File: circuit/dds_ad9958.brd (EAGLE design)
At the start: 84 x 40.5 mm, 68 parts, among them IC1 TPS76833, IC2 TPS79318, IC3 TPS79318, IC4 AD9958, Q1 25MHz, X2 BU-SMA-V, X3 BU-SMA-V

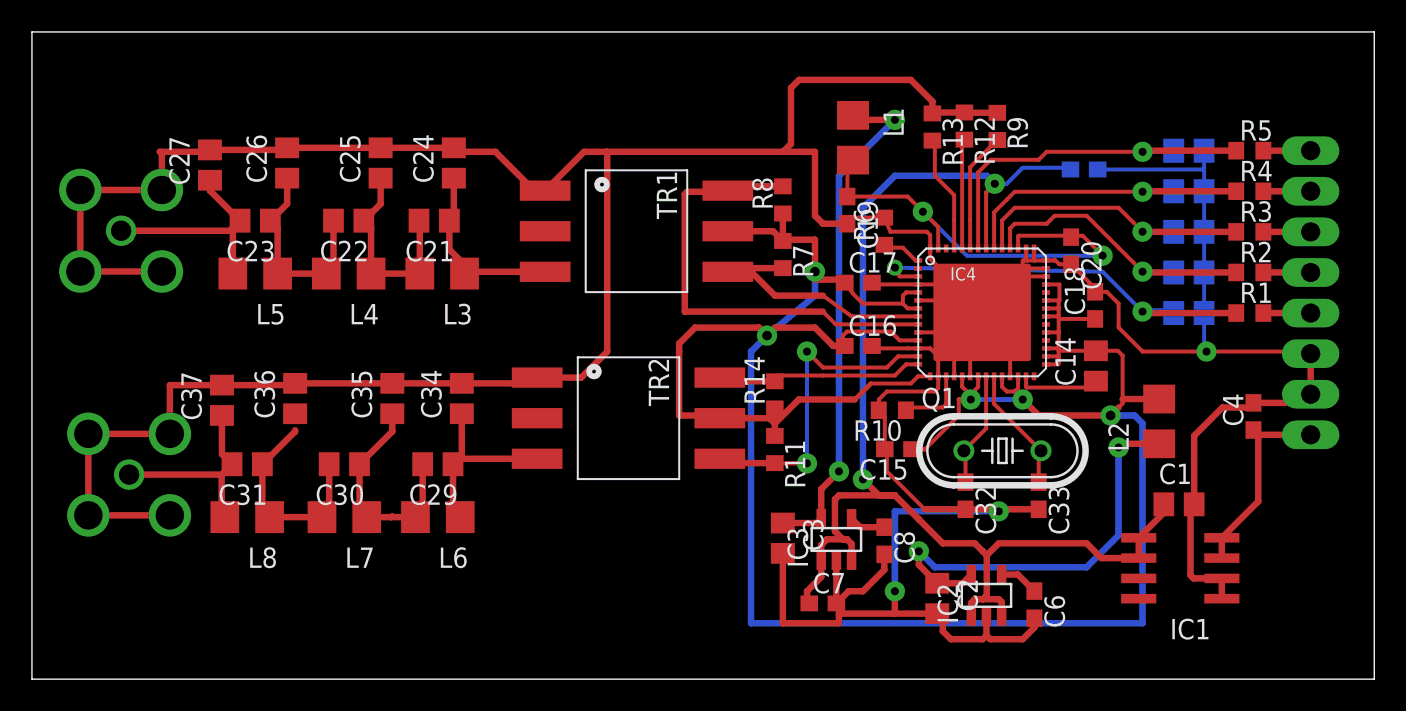
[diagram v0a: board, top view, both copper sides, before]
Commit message: - ??????? ? ????????? ????????
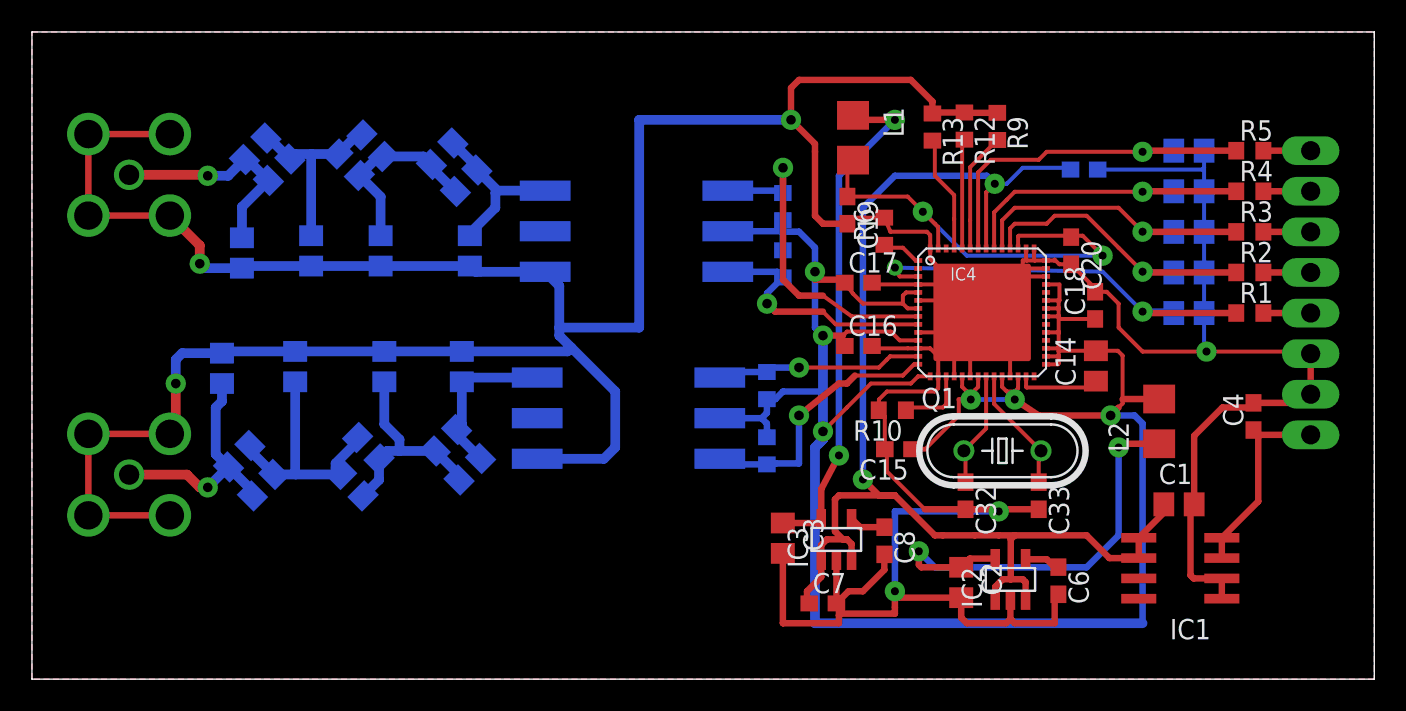
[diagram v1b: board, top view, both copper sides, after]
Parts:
- L3, L4, L5, L6, L7, L8: device rcl:L3225P -> rcl:C0805
- moved L4 8.14 mm to (21.3, 33.4), flipped to the bottom, turned to 45 degrees
- moved L3 7.50 mm to (25.7, 32.9), flipped to the bottom, turned to 315 degrees
- moved L5 6.67 mm to (15.5, 31.9), flipped to the bottom, turned to 315 degrees
- moved C27 5.85 mm to (13.1, 26.7), flipped to the bottom, turned to 270 degrees
- moved C26 5.70 mm to (17.5, 26.8), flipped to the bottom, turned to 270 degrees
- moved C24 5.59 mm to (27.4, 26.8), flipped to the bottom, turned to 270 degrees
- moved C25 5.50 mm to (21.8, 26.8), flipped to the bottom, turned to 270 degrees
- moved C23 4.50 mm to (14.0, 33.2), flipped to the bottom, turned to 315 degrees
- moved R11 4.03 mm to (46.0, 18.4), flipped to the bottom, turned to 90 degrees
- moved R8 4.00 mm to (47.0, 26.0), flipped to the bottom, turned to 270 degrees
- moved L6 3.61 mm to (27.4, 13.1), flipped to the bottom, turned to 315 degrees
- moved R14 3.54 mm to (46.0, 14.3), flipped to the bottom, turned to 270 degrees
- moved X2 3.54 mm to (6.08, 31.6)
- moved C22 3.50 mm to (19.8, 32.2), flipped to the bottom, turned to 45 degrees
- moved C21 3.20 mm to (27.2, 31.2), flipped to the bottom, turned to 315 degrees
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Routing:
- net AVDD: track 168.3 -> 145.9 mm, vias 5 -> 6
- net GND: track 328.7 -> 342.5 mm, vias 3 -> 6
- net N$7: track 28.6 -> 15.6 mm, vias 0 -> 1
- net N$9: track 20.2 -> 13.0 mm, vias 2 -> 1
- net N$3: track 16.5 -> 21.4 mm, vias 0 -> 1
- net N$10: track 12.9 -> 16.8 mm, vias 0 -> 1
- net N$26: track 12.8 -> 15.2 mm, vias 0 -> 1
- net N$25: track 13.3 -> 15.5 mm
- net N$23: track 12.3 -> 10.4 mm
- net N$11: track 13.0 -> 11.8 mm
- net N$6: track 26.7 -> 27.8 mm
- net N$2: track 11.6 -> 10.5 mm
- net N$18: track 13.1 -> 12.3 mm
- net N$24: track 14.1 -> 13.6 mm
- net N$20: track 13.9 -> 14.0 mm, vias 0 -> 1
- added copper zone on layer 1, net GND
- added copper zone on layer 16, net GND
